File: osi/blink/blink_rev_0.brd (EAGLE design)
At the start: 25.4 x 25.4 mm, 4 parts

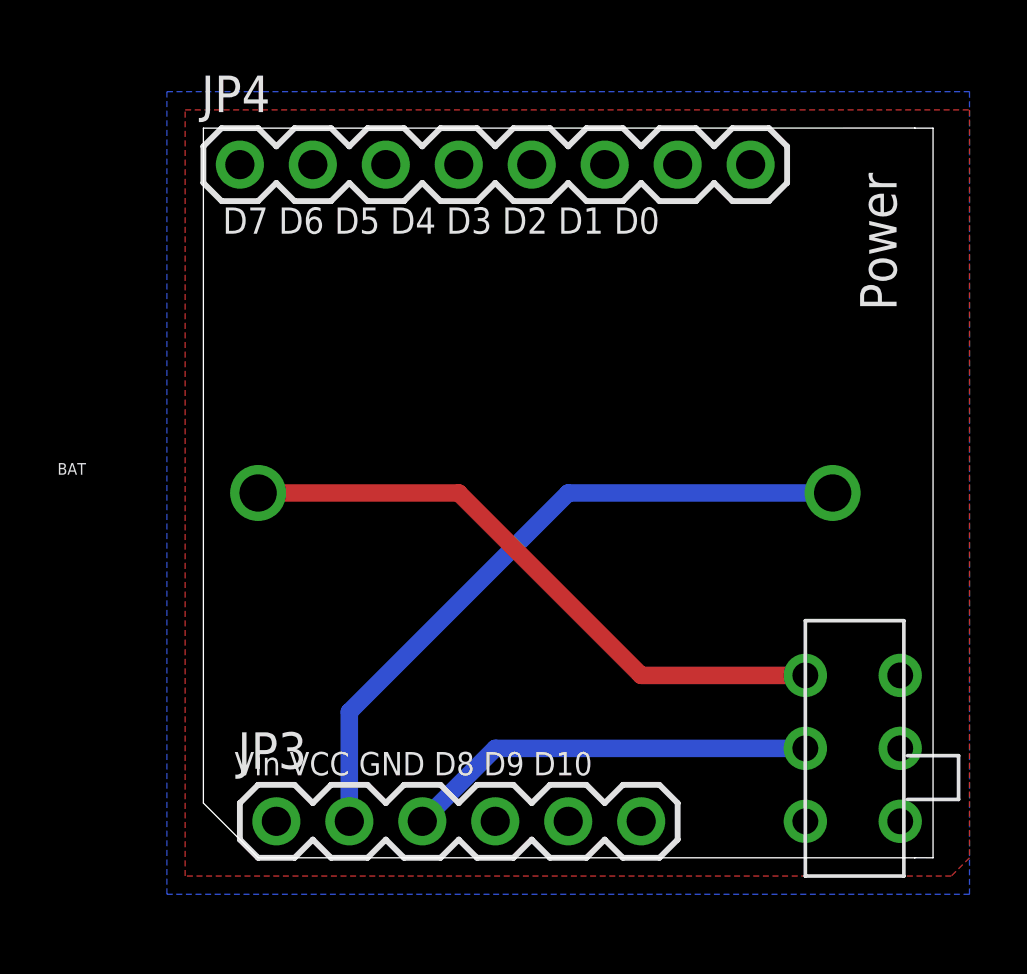
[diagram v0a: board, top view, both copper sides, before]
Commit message: update
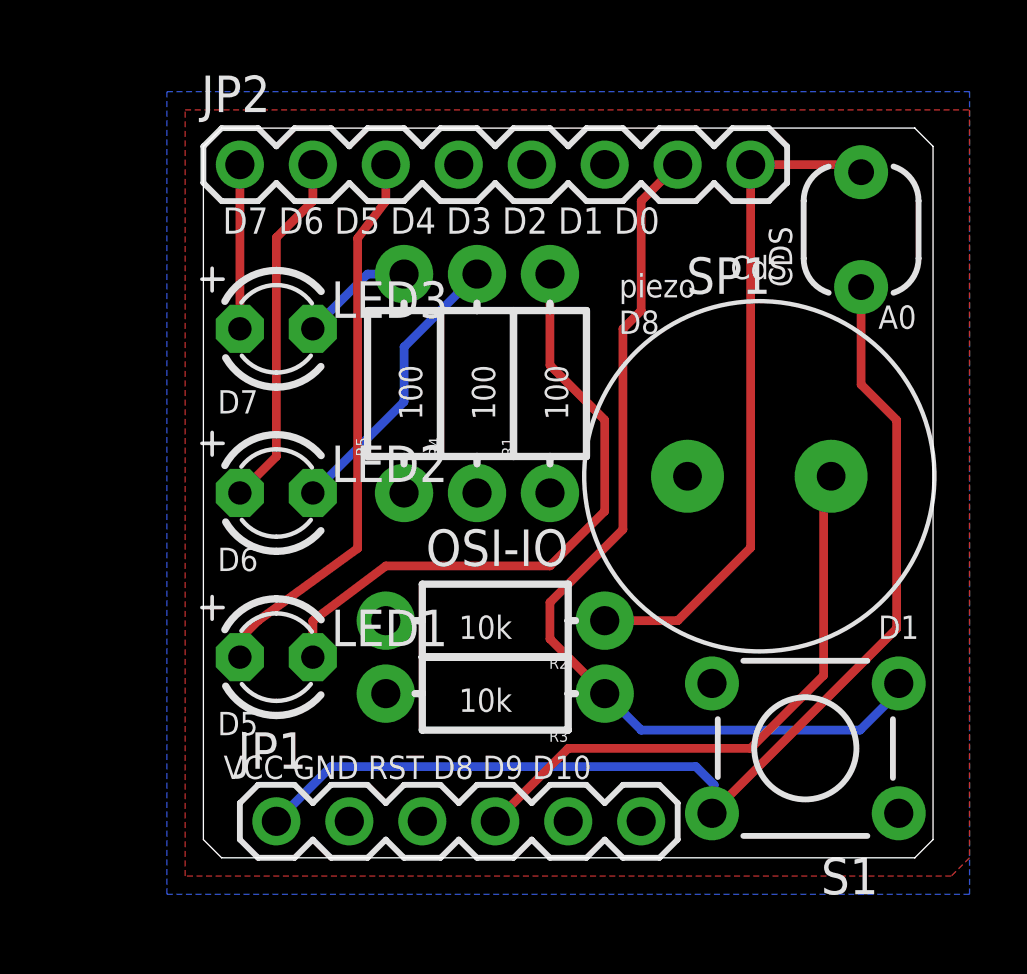
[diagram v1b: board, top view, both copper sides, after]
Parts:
- removed BAT: (no value), SparkFun_mod:BATTCOM_20MM_PTH
- removed U$1: SWITCH, _my-parts:SWITCH
- added CDS: PHOTOCELLPTH-KIT, SparkFun_mod:PHOTOCELL-KIT
- added LED1, LED2, LED3: (no value), adafruit:LED3MM
- added R1, R2, R3, R4, R5: (no value), SparkFun_mod:AXIAL-0.3-KIT
- added S1: (no value), SparkFun_mod:TACTILE-PTH
- added SP1: SPEAKER/PS12, adafruit_mod:PS12
- renumbered JP3 to JP1, JP4 to JP2
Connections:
- removed net V+: JP1.1
- new net N$2: LED2.K, R4.P$2
- new net N$3: LED3.K, R5.P$2
- new net RESET: JP1.3
- net D0: now also CDS.2, R2.P$1
- net D1: now also R3.P$1, S1.3
- net D5: now also LED1.A
- net D6: now also LED2.A
- net D7: now also LED3.A
- net D8: now also SP1.P$2
- net GND: now also JP1.2, R1.P$1, R2.P$2, R3.P$2, R4.P$1, R5.P$1, SP1.P$1; no longer JP1.3, U$1.2
- net N$1: now also LED1.K, R1.P$2; no longer BAT.2, U$1.3
- net VCC: now also CDS.1, JP1.1, S1.2; no longer BAT.1, JP1.2
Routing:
- net D1: track 0.00 -> 32.6 mm
- net D0: track 0.00 -> 23.4 mm
- net D8: track 0.00 -> 20.6 mm
- net D5: track 0.00 -> 19.5 mm
- net VCC: track 23.8 -> 38.8 mm
- net GND: track 14.4 -> 0.00 mm
- net D6: track 0.00 -> 12.5 mm
- net N$2: track 0.00 -> 9.99 mm
- net D7: track 0.00 -> 5.71 mm
- net N$3: track 0.00 -> 3.96 mm
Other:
- outline, holes or cut-outs redrawn
- board text added: "100"
- board text added: "10k"
- board text added: "A0"
- board text added: "CdS"
- board text added: "D1"
- board text added: "D5"
- board text added: "D6"
- board text added: "D7"
- board text added: "D8"
- board text added: "MakersBox.blogspot.com"
- board text added: "OSI-IO"
- board text added: "VCC GND RST D8 D9 D10"
- board text added: "piezo"
- board text removed: "CR2032"
- board text removed: "Power"
- board text removed: "Vin VCC GND D8 D9 D10"
- board text removed: "makersbox.blogspot.com"
